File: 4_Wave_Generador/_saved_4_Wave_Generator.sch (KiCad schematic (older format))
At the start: 121 parts, among them J1 RS232, J10 Jumper, J11 Jumper, J12 Jumper, J13 Jumper, J14 Jumper, J15 Jumper, J2 I2C, J3 RS232_PIC, J4 RESET, J5 Jumper, J7 Jumper, P1 ECG INPUTS, P10 INPUT_ADC_PIC, P11 IN_MUX1, P12 RG_8421, P13 IN_MUX2, P14 OUTPUT_TARJET, P15 OUTPUT_DIG_PIC, P16 OUTPUT_DIG_ATMEGA328P, P17 5 V, P2 PIC_PROGRAMER, P3 SPI_MICRO, P4 AD8232_CONTROL, P5 OXIMETRO, P6 GND, P7 CONN_01X04, P8 MCLK_EXTERNAL, P9 SPI_AD9833, SW1 SW_Push, SW2 RESET_PIC, U1 PIC16F688, U2 AD8232_A, U3 ATMEGA328P-AU_MIO, U4 AD9833, U5 LD1117S33TR_MIO, U6 ADG819, U7 ADG819, U8 AD8421, Y1 Crystal_8MHz, Y2 XRCHA_16M

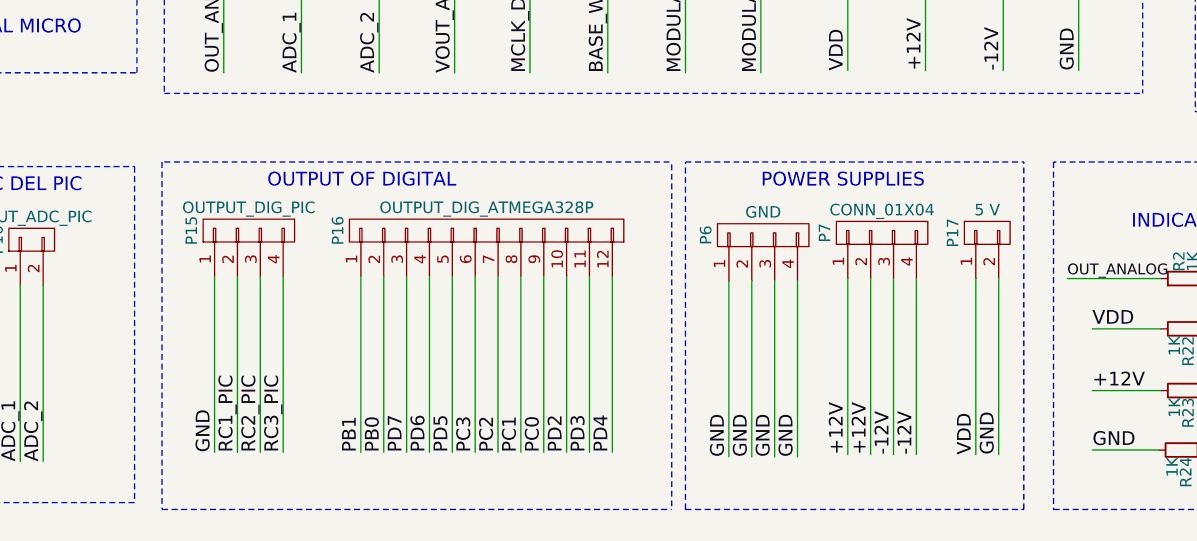
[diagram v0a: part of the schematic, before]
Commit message: GENERADOR_V8
ORGANIZACION DE ELEMENTOS
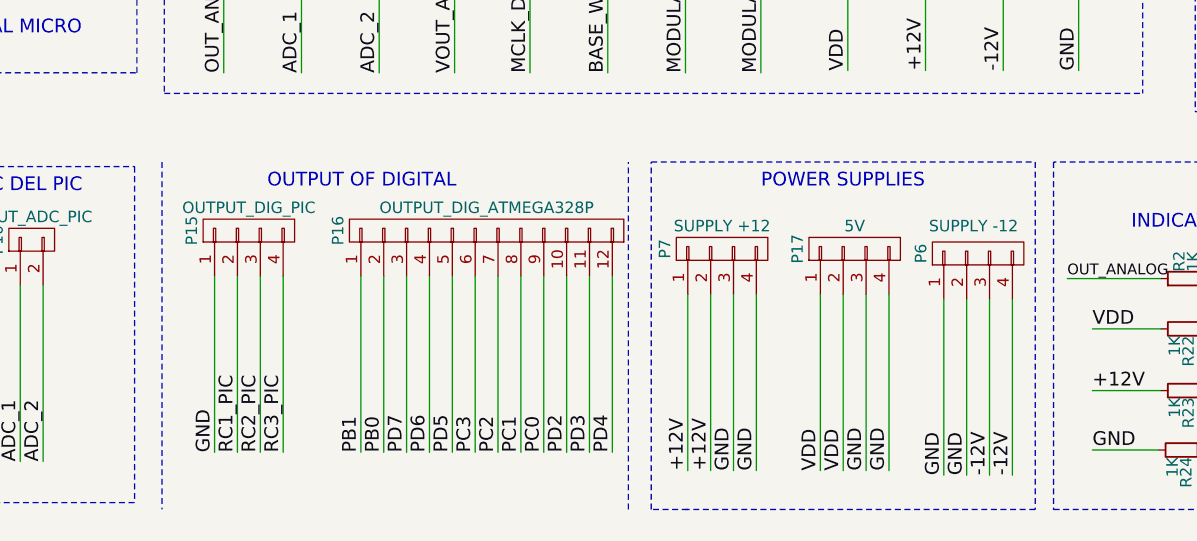
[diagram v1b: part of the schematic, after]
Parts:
- removed P17: 5 V, Foot_Prints_Manager_Outputs:5V, symbol CONN_01X02
- added P17: 5V, Foot_Prints_Manager_Outputs:SUPPLY_5V, symbol CONN_01X04
- P16: footprint Pin_Headers:Pin_Header_Straight_1x12_Pitch2.54mm -> Foot_Prints_Manager_Outputs:OUTPUT_ATMEGA
- P6: value GND -> SUPPLY -12; footprint Pin_Headers:Pin_Header_Straight_1x04_Pitch2.54mm -> Foot_Prints_Manager_Outputs:SUPPLY_-12V
- P7: value CONN_01X04 -> SUPPLY +12; footprint Pin_Headers:Pin_Header_Angled_1x04_Pitch2.54mm -> Foot_Prints_Manager_Outputs:SUPPLY_12V
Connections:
- net -12V: now also P6.3 (P3), P6.4 (P4); no longer P7.3 (P3), P7.4 (P4)
- net GND: now also P7.3 (P3), P7.4 (P4), P17.3 (P3), P17.4 (P4); no longer P6.3 (P3), P6.4 (P4)
- net VDD: now also P17.1 (P1), P17.2 (P2)
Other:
- moved on the sheet: P6, P7
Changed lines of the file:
@@
 Text Label 15280 6550 1    60   ~ 0
 MODULATED_WAVE_1
-Text Label 9100 10890 1    60   ~ 0
+Text Label 9840 10970 1    60   ~ 0
 GND
 Text Label 10490 10330 0    60   ~ 0
@@
 L CONN_01X04 P6
 U 1 1 59D306D3
-P 9050 9920
-F 0 "P6" H 9050 10170 50  0000 C CNN
-F 1 "GND" V 9150 9920 50  0000 C CNN
-F 2 "Pin_Headers:Pin_Header_Straight_1x04_Pitch2.54mm" H 9050 9920 50  0001 C CNN
-F 3 "" H 9050 9920 50  0000 C CNN
-	1    9050 9920
-	0    -1   -1   0
-$EndComp
-Text Label 9200 10890 1    60   ~ 0
-GND
-Text Label 9720 10880 1    60   ~ 0
--12V
+P 9990 10000
+F 0 "P6" H 9990 10250 50  0000 C CNN
+F 1 "SUPPLY -12" V 10110 10020 50  0000 C CNN
+F 2 "Foot_Prints_Manager_Outputs:SUPPLY_-12V" H 9990 10000 50  0001 C CNN
+F 3 "" H 9990 10000 50  0000 C CNN
+	1    9990 10000
+	0    -1   -1   0
+$EndComp
+Text Label 9940 10970 1    60   ~ 0
+GND
+Text Label 9020 10950 1    60   ~ 0
+GND
 $Comp
 L CONN_01X04 P7
 U 1 1 59D306D4
-P 9570 9910
-F 0 "P7" H 9570 10160 50  0000 C CNN
-F 1 "CONN_01X04" V 9670 9910 50  0000 C CNN
-F 2 "Pin_Headers:Pin_Header_Angled_1x04_Pitch2.54mm" H 9570 9910 50  0001 C CNN
-F 3 "" H 9570 9910 50  0000 C CNN
-	1    9570 9910
-	0    -1   -1   0
-$EndComp
-Text Label 9620 10880 1    60   ~ 0
--12V
-Text Label 9520 10880 1    60   ~ 0
+P 8870 9980
+F 0 "P7" H 8870 10230 50  0000 C CNN
+F 1 "SUPPLY +12" V 8970 9980 50  0000 C CNN
+F 2 "Foot_Prints_Manager_Outputs:SUPPLY_12V" H 8870 9980 50  0001 C CNN
+F 3 "" H 8870 9980 50  0000 C CNN
+	1    8870 9980
+	0    -1   -1   0
+$EndComp
+Text Label 8920 10950 1    60   ~ 0
+GND
+Text Label 8820 10950 1    60   ~ 0
 +12V
-Text Label 9420 10880 1    60   ~ 0
+Text Label 8720 10950 1    60   ~ 0
 +12V
 Text Label 8950 2150 2    60   ~ 0
@@
 $EndComp
 Text Label 11660 10110 2    60   ~ 0
-GND
-Text Label 9000 10890 1    60   ~ 0
-GND
-Text Label 8900 10890 1    60   ~ 0
 GND
 Text Label 14420 8690 1    60   ~ 0
@@
 Wire Notes Line
 	15840 890  15840 1750
-Wire Notes Line
-	8650 9610 8650 11120
 Wire Wire Line
 	6690 8360 6690 9210
@@
 	10430 8350 10430 9200
 Wire Wire Line
-	8900 10120 8900 10890
-Wire Wire Line
-	9000 10120 9000 10890
-Wire Wire Line
-	9100 10120 9100 10890
-Wire Wire Line
-	9200 10120 9200 10890
-Wire Wire Line
-	9420 10110 9420 10880
-Wire Wire Line
-	9520 10110 9520 10880
-Wire Wire Line
-	9620 10110 9620 10880
-Wire Wire Line
-	9720 10110 9720 10880
-Wire Notes Line
-	8710 9600 10190 9600
-Wire Notes Line
-	8710 11120 10190 11120
-Wire Notes Line
-	8710 11120 8710 9600
+	9840 10200 9840 10970
+Wire Wire Line
+	9940 10200 9940 10970
+Wire Wire Line
+	10040 10200 10040 10970
+Wire Wire Line
+	10140 10200 10140 10970
+Wire Wire Line
+	8720 10180 8720 10950
+Wire Wire Line
+	8820 10180 8820 10950
+Wire Wire Line
+	8920 10180 8920 10950
+Wire Wire Line
+	9020 10180 9020 10950
+Wire Notes Line
+	8560 9600 10240 9600
+Wire Notes Line
+	10240 11120 8710 11120
 Wire Notes Line
 	6430 7880 6430 9300
@@
 F 0 "P16" H 7840 10550 50  0000 C CNN
 F 1 "OUTPUT_DIG_ATMEGA328P" V 7940 9900 50  0000 C CNN
-F 2 "Pin_Headers:Pin_Header_Straight_1x12_Pitch2.54mm" H 7840 9900 50  0001 C CNN
+F 2 "Foot_Prints_Manager_Outputs:OUTPUT_ATMEGA" H 7840 9900 50  0001 C CNN
 F 3 "" H 7840 9900 50  0000 C CNN
 	1    7840 9900
@@
 	5330 11080 2040 11080
 Wire Notes Line
-	8640 9600 6420 9600
-Wire Notes Line
 	6420 9600 6420 11120
-Wire Notes Line
-	6420 11120 8650 11120
 $Comp
 L CONN_01X02 P10
@@
 Wire Notes Line
 	2040 11080 2040 9620
-$Comp
-L CONN_01X02 P17
-U 1 1 59D951A4
-P 10030 9910
-F 0 "P17" H 10030 10060 50  0000 C CNN
-F 1 "5 V" V 10130 9910 50  0000 C CNN
-F 2 "Foot_Prints_Manager_Outputs:5V" H 10030 9910 50  0001 C CNN
-F 3 "" H 10030 9910 50  0000 C CNN
-	1    10030 9910
-	0    -1   -1   0
-$EndComp
-Wire Wire Line
-	9980 10110 9980 10880
-Wire Wire Line
-	10080 10110 10080 10880
-Text Label 9980 10880 1    60   ~ 0
+Wire Wire Line
+	9400 10180 9400 10950
+Wire Wire Line
+	9500 10180 9500 10950
+Text Label 9400 10950 1    60   ~ 0
 VDD
-Text Label 10080 10880 1    60   ~ 0
-GND
-Wire Notes Line
-	10190 11120 10190 9600
+Text Label 9500 10950 1    60   ~ 0
+GND
+Wire Notes Line
+	10240 9600 10240 11120
 Wire Notes Line
 	10320 9600 10320 11120
@@
 	0    1    1    0
 $EndComp
+Text Label 10040 10970 1    60   ~ 0
+-12V
+Text Label 10140 10970 1    60   ~ 0
+-12V
+Wire Notes Line
+	8460 11120 8460 9600
+$Comp
+L CONN_01X04 P17
+U 1 1 59E75390
+P 9450 9980
+F 0 "P17" H 9450 10230 50  0000 C CNN
+F 1 "5V" V 9550 9980 50  0000 C CNN
+F 2 "Foot_Prints_Manager_Outputs:SUPPLY_5V" H 9450 9980 50  0001 C CNN
+F 3 "" H 9450 9980 50  0000 C CNN
+	1    9450 9980
+	0    -1   -1   0
+$EndComp
+Wire Notes Line
+	8720 11120 8560 11120
+Wire Notes Line
+	8560 11120 8560 9600
+Wire Wire Line
+	9300 10180 9300 10950
+Text Label 9300 10950 1    60   ~ 0
+VDD
+Wire Wire Line
+	9600 10180 9600 10950
+Text Label 9600 10950 1    60   ~ 0
+GND
 $EndSCHEMATC
